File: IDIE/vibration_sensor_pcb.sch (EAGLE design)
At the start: 63 parts, among them IC1 LORA-E5, IC2 STM32L071KBT6, IC3 FXLS8974CFR3, IC4 FXLS8971CFR1, IC5 DRV5032FBLPGM, IC6 FT234XD-T, J1 217182-0001, Q2 SI2305B-TP, Y1 ABS06-32.768KHZ-9-1-T

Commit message: ADD & UPDATE documentacion, modelado 3d y poco ruteo
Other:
- note added: "Diodo Protexion"
- note added: "Filtro"
- note added: "Filtro Bus"
- note added: "Led RGB"
- note added: "Modulo LoRa"
- note added: "Modulo Serial"
- note added: "Procesador"
- note added: "Puntos Guia"
- note added: "SANTIAGO CORTÉS TOVAR ANTHONY DE JESUS G"
- note added: "Selectores de uso"
- note added: "Sensor Efecto Tunel"
- note added: "Sensor Triaxial"
- note added: "Socket y protección"
- note added: "USB type C"
- note removed: "ESCUELA COLOMBIANA DE INGENIERIA"
- moved on the sheet: ANT1, C1, C10, C11, C12, C13, C14, C15, C16, C17, C18, C2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

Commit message: UPDATE schematic
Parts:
- removed D1: SP0503BAHTG, SamacSys_Parts:SP0503BAHTG
- added IC7: USBLC6-2SC6, SamacSys_Parts:USBLC6-2SC6
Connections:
- removed net SCL: JMP2-0R.3
- removed net SDA: JMP1-0R.3
- new net N$10: IC7.I/O2_1
- new net N$3: IC7.I/O1_2
- new net N$4: IC7.I/O2_2
- new net N$7: IC7.I/O1_1
- net GND: now also IC7.GND; no longer D1.COMMON_A
- net I2C_SCL: now also JMP2-0R.3
- net I2C_SDA: now also JMP1-0R.3
- net USB_N: no longer D1.K_2
- net USB_P: no longer D1.K_1
- net VBUS: now also IC7.VBUS; no longer D1.K_3
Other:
- note removed: "Diodo Protexion"
- note removed: "Filtro"
- note removed: "Filtro Bus"
- note removed: "Led RGB"
- note removed: "Modulo LoRa"
- note removed: "Modulo Serial"
- note removed: "Procesador"
- note removed: "Puntos Guia"
- note removed: "Selectores de uso"
- note removed: "Sensor Efecto Tunel"
- note removed: "Sensor Triaxial"
- note removed: "Socket y protección"
- note removed: "USB type C"
- moved on the sheet: ANT1, C1, C10, C11, C12, C13, C14, C15, C16, C17, C18, C2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

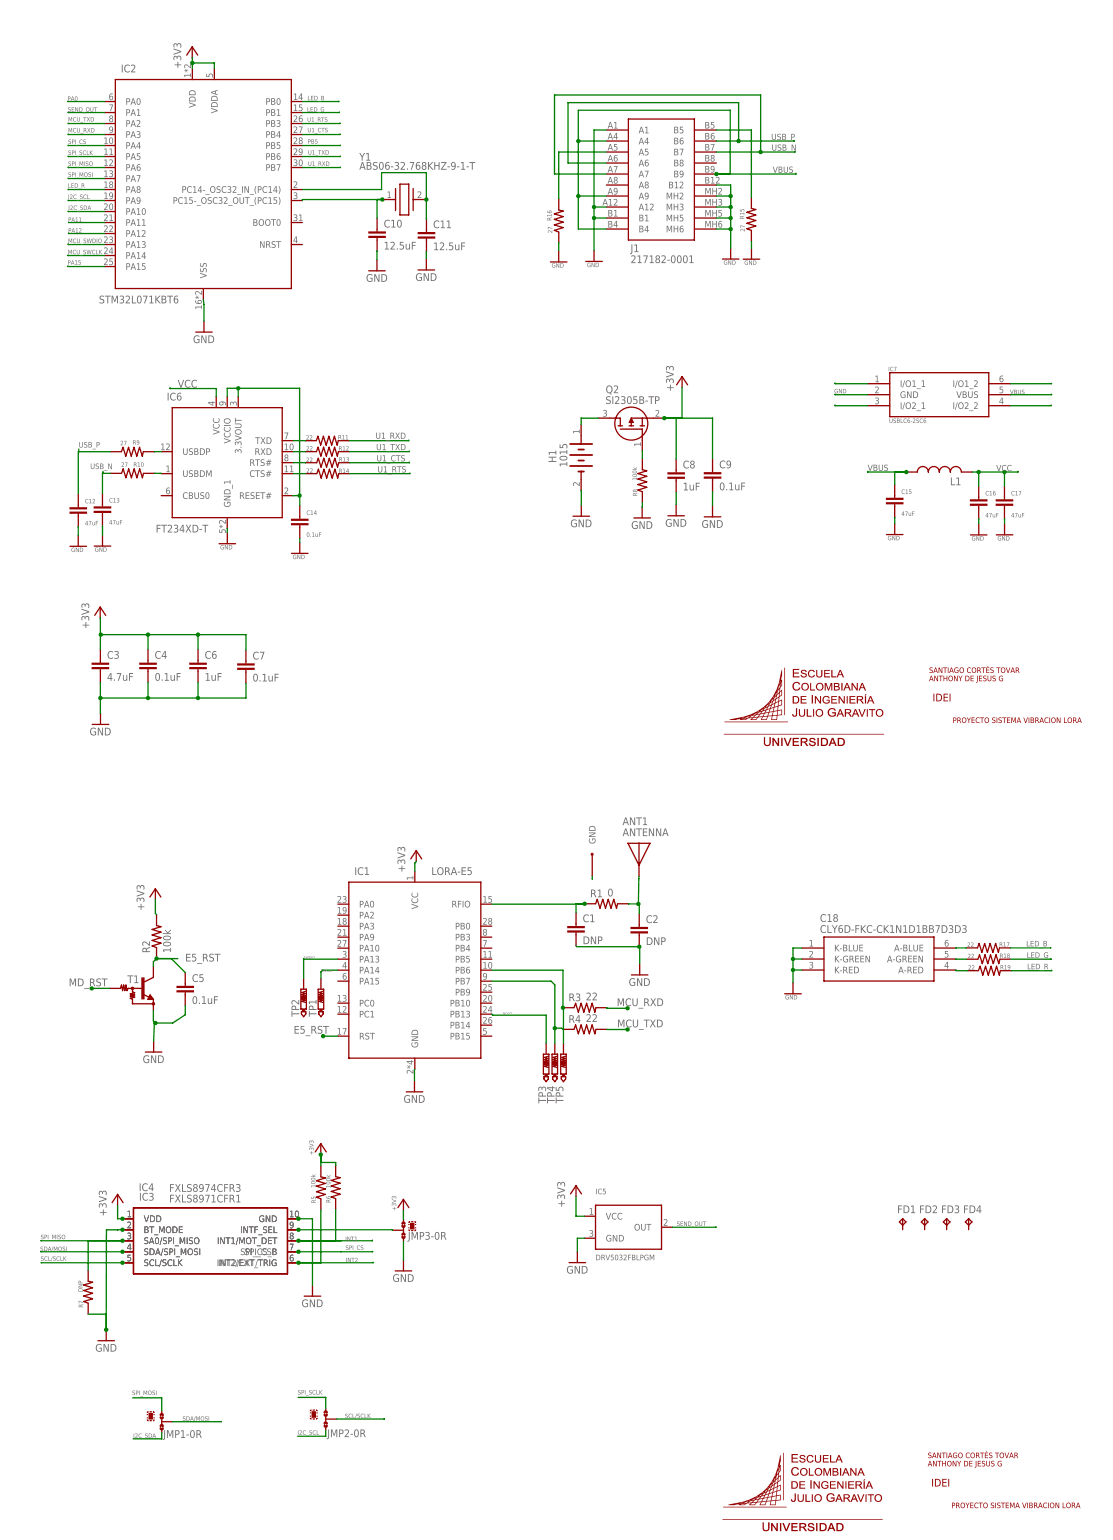
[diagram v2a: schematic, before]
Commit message: UPDATE schematic and PCB route
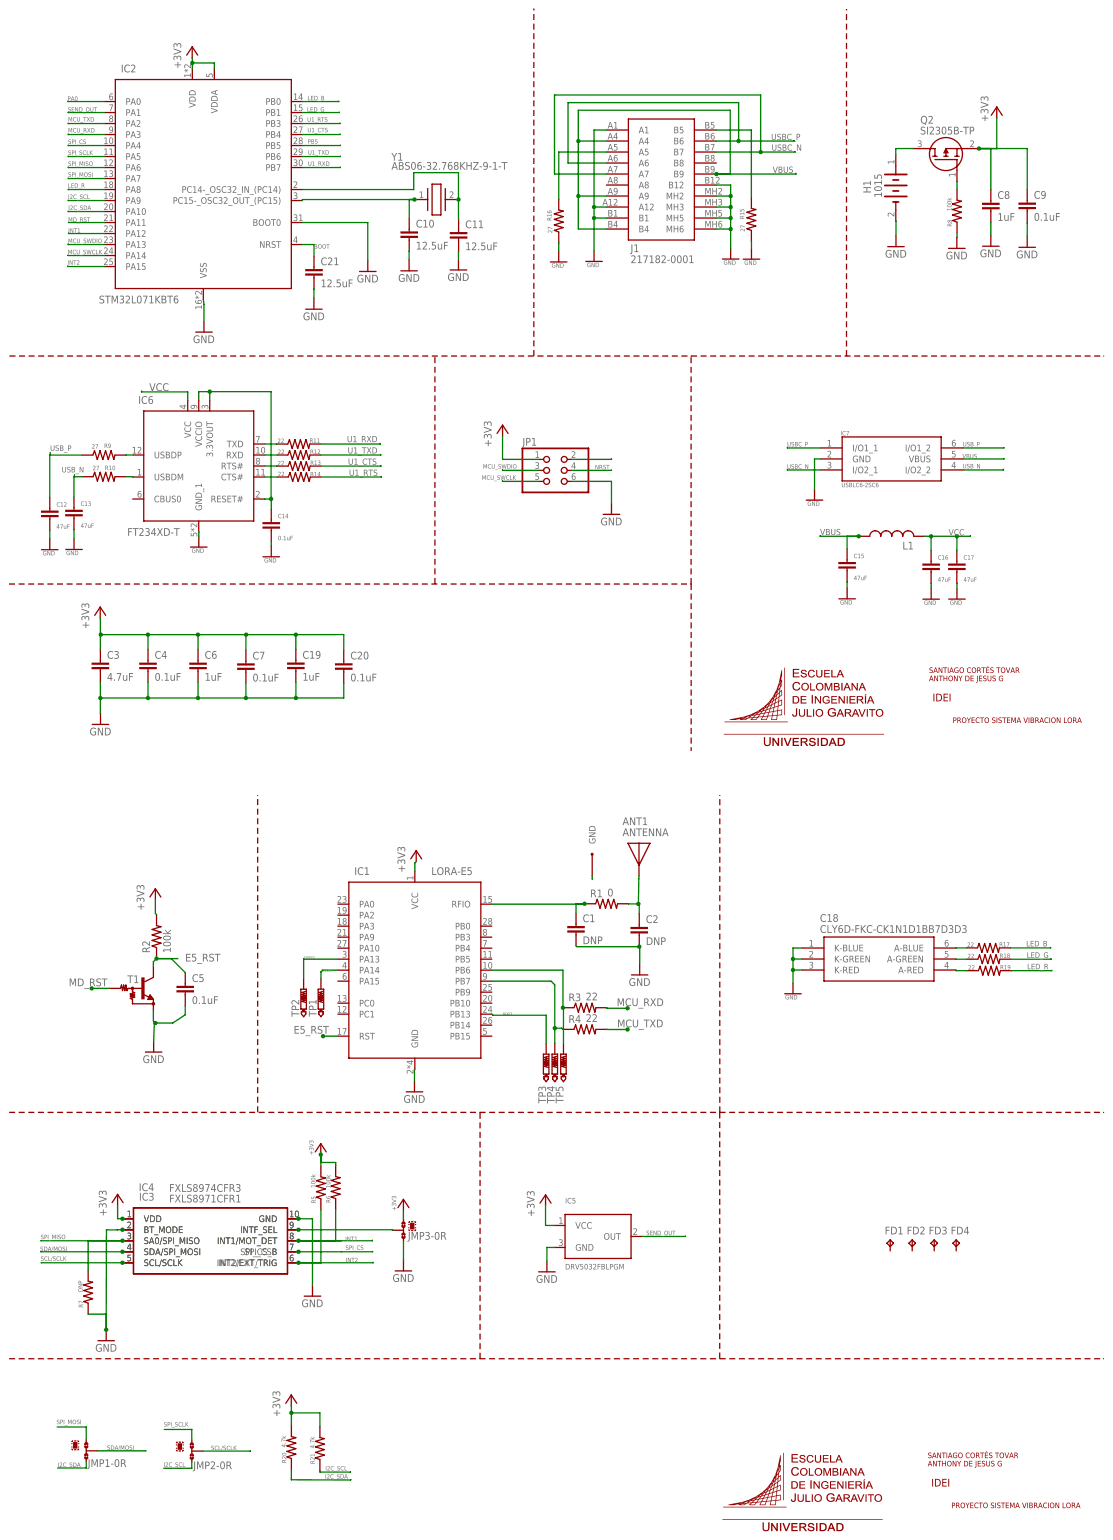
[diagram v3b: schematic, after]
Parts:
- added C19: 1uF, rcl:C-EUC0603
- added C20: 0.1uF, rcl:C-EUC0603
- added C21: 12.5uF, rcl:C-EUC0603
- added JP1: (no value), pinhead:PINHD-2X3
- added R20, R21: 4.7k, rcl:R-US_R0603
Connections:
- net N$1 renamed INTF_SEL
- net N$9 renamed RESET#
- removed net N$10: IC7.I/O2_1
- removed net N$3: IC7.I/O1_2
- removed net N$4: IC7.I/O2_2
- removed net N$7: IC7.I/O1_1
- removed net PA11: IC2.PA11
- removed net PA12: IC2.PA12
- removed net PA15: IC2.PA15
- new net GND1: C20.2
- new net N$2: JP1.2
- new net NRST: JP1.4
- new net USBC_N: IC7.I/O2_1, J1.A7, J1.B7
- new net USBC_P: IC7.I/O1_1, J1.A6, J1.B6
- net +3V3: now also C19.1, C20.1, JP1.1, R20.2, R21.2
- net BOOT: now also C21.1, IC2.NRST
- net GND: now also C19.2, C21.2, IC2.BOOT0, JP1.6
- net I2C_SCL: now also R21.1
- net I2C_SDA: now also R20.1
- net INT1: now also IC2.PA12
- net INT2: now also IC2.PA15
- net MCU_SWCLK: now also JP1.5
- net MCU_SWDIO: now also JP1.3
- net MD_RST: now also IC2.PA11
- net USB_N: now also IC7.I/O2_2; no longer J1.A7, J1.B7
- net USB_P: now also IC7.I/O1_2; no longer J1.A6, J1.B6
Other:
- moved on the sheet: C10, C11, C12, C13, C14, C15, C16, C17, C8, C9, FD1, FD2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

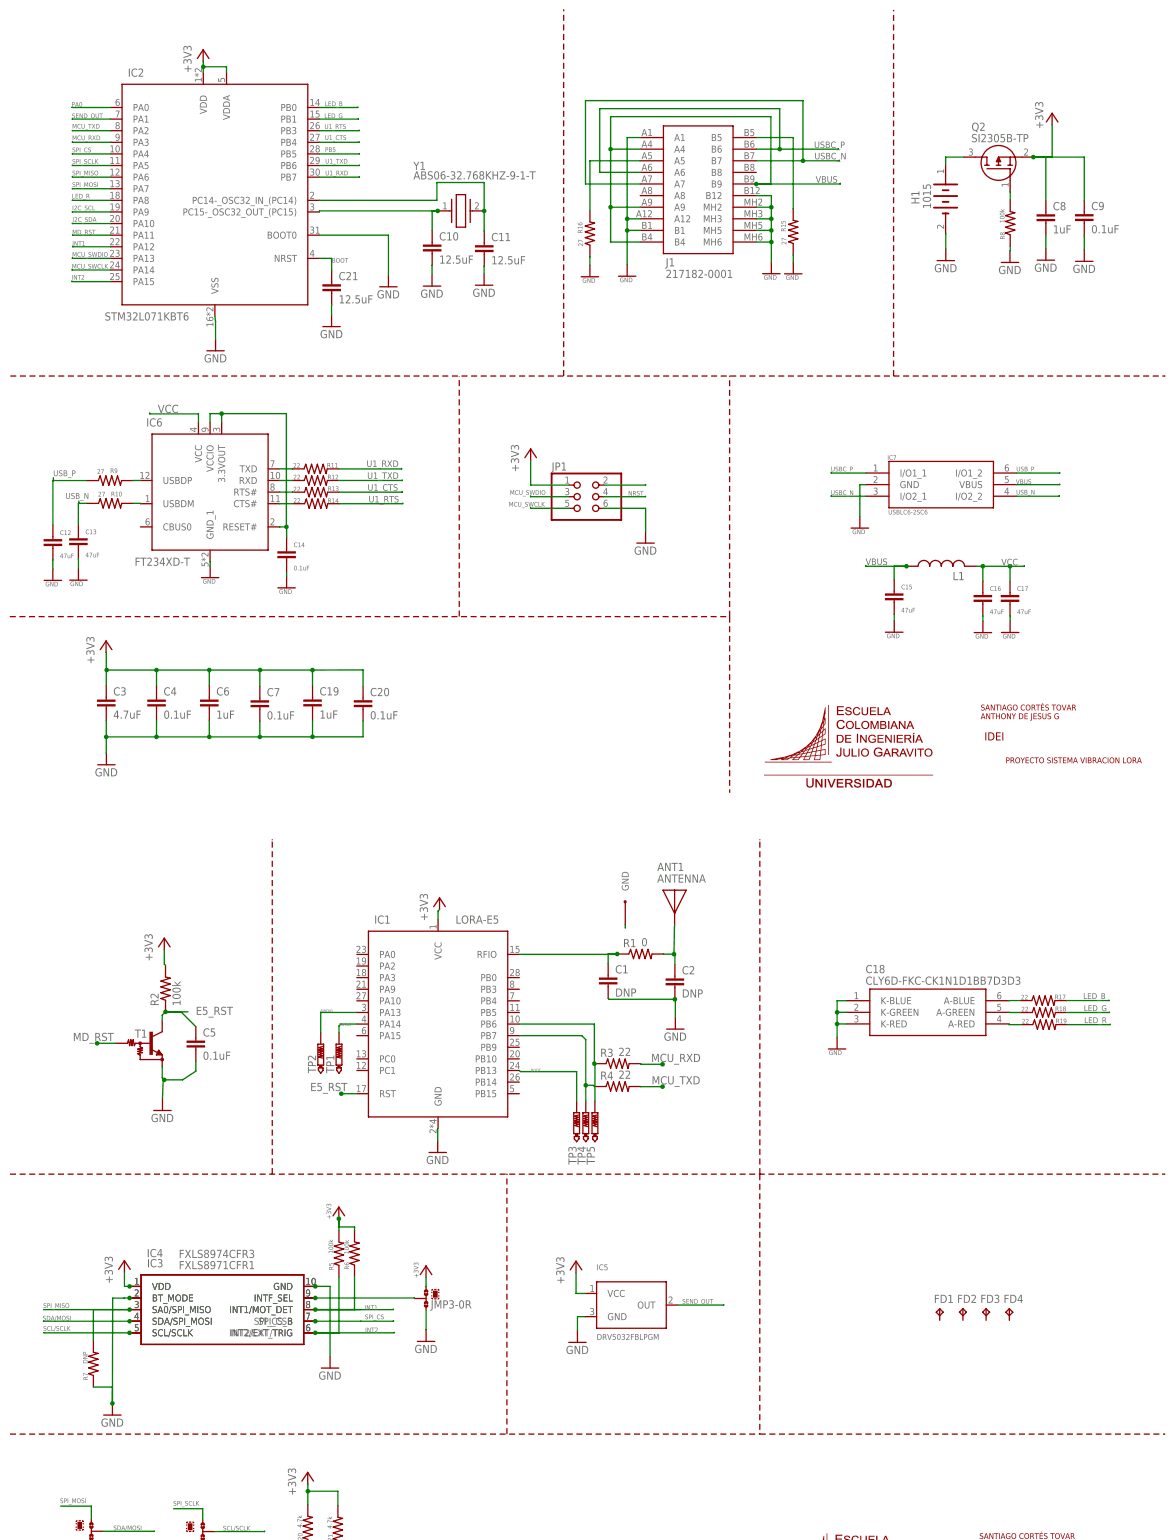
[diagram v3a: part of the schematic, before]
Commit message: UPDATE pcb schematic
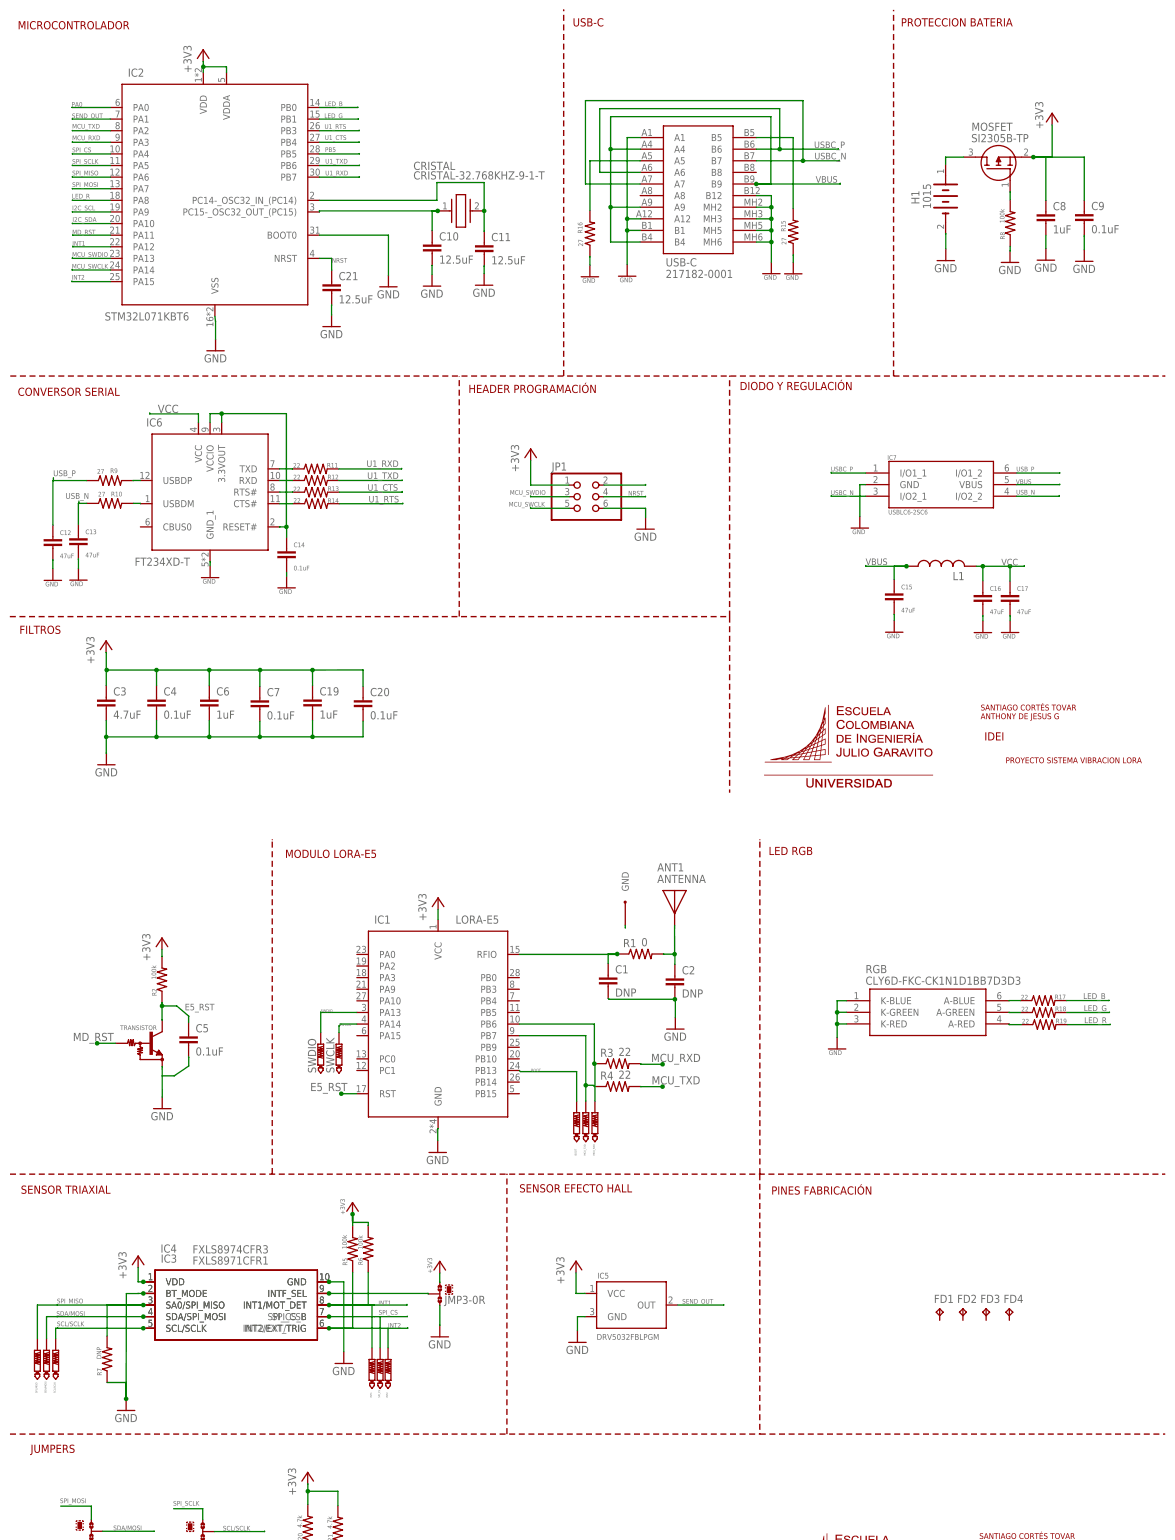
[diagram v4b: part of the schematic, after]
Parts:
- removed Y1: ABS06-32.768KHZ-9-1-T, SamacSys_Parts:ABS06-32.768KHZ-9-1-T
- added CRISTAL: CRISTAL-32.768KHZ-9-1-T, SamacSys_Parts:CRISTAL-32.768KHZ-9-1-T
- added INT1, INT2, SCL/SCLK, SDA/MOSI, SPI_CS, SPI_MISO: PTR1TP11R, testpad:PTR1TP11R
- renumbered C18 to RGB, J1 to USB-C, Q2 to MOSFET, T1 to TRANSISTOR, TP1 to SWCLK, TP2 to SWDIO, TP3 to BOOT, TP4 to MCU_TXD, TP5 to MCU_RXD
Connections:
- net N$6 renamed GATE
- net BOOT: no longer C21.1, IC2.NRST
- net INT1: now also INT1.TP
- net INT2: now also INT2.TP
- net NRST: now also C21.1, IC2.NRST
- net OSC32_IN: now also CRISTAL.2; no longer Y1.2
- net OSC32_OUT: now also CRISTAL.1; no longer Y1.1
- net SCL/SCLK: now also SCL/SCLK.TP
- net SDA/MOSI: now also SDA/MOSI.TP
- net SPI_CS: now also SPI_CS.TP
- net SPI_MISO: now also SPI_MISO.TP
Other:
- note added: "CONVERSOR SERIAL"
- note added: "DIODO Y REGULACIÓN"
- note added: "FILTROS"
- note added: "HEADER PROGRAMACIÓN"
- note added: "JUMPERS"
- note added: "LED RGB"
- note added: "MICROCONTROLADOR"
- note added: "MODULO LORA-E5"
- note added: "PINES FABRICACIÓN"
- note added: "PROTECCION BATERIA"
- note added: "SENSOR EFECTO HALL"
- note added: "SENSOR TRIAXIAL"
- note added: "USB-C"
- moved on the sheet: C5, IC3, IC4, JMP3-0R, R2, R5, R6, R7
